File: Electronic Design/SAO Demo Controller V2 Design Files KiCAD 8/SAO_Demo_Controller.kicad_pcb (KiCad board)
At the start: 2 copper layers, 38.1 x 50.8 mm, 10 parts, among them U1 RP2040-Zero, X1 SAO_conn, X2 SAO_conn, X5 QWIIC, X6 QWIIC

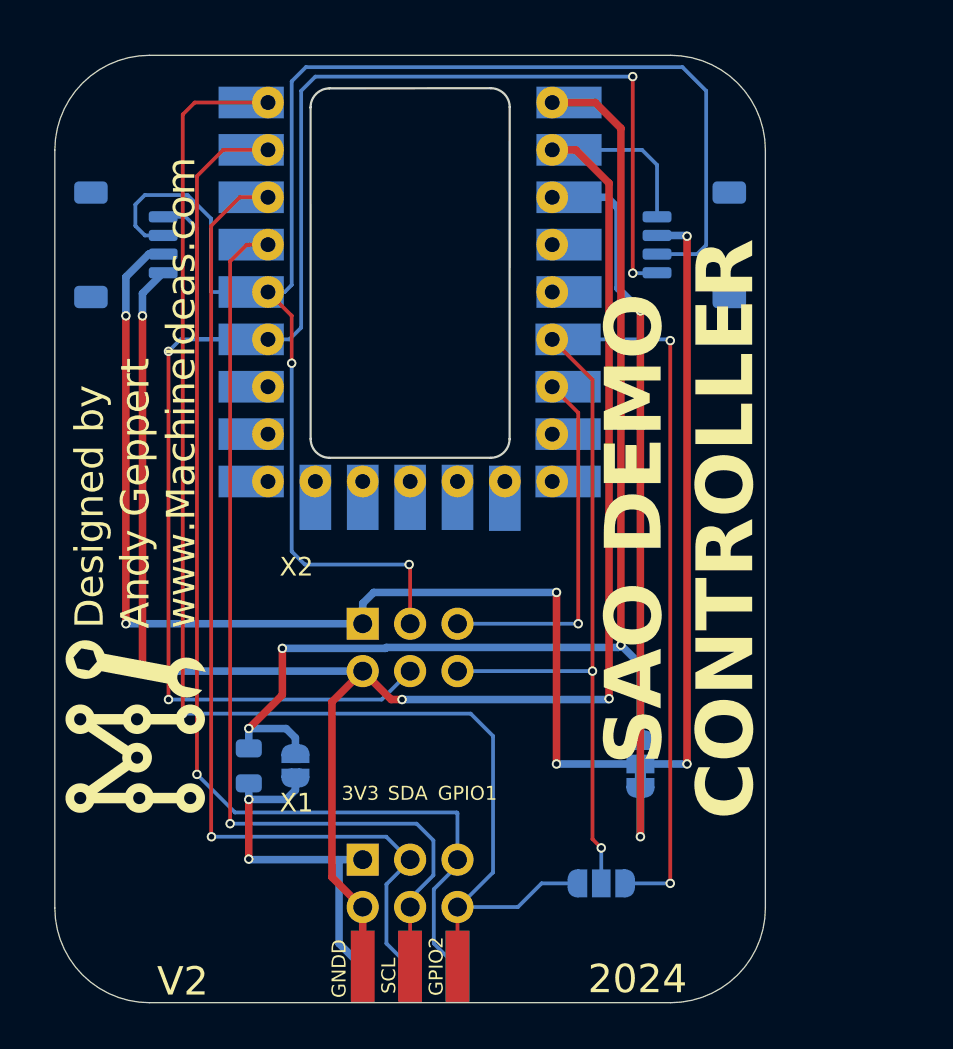
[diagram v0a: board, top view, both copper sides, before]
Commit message: Update V2 schematics, docs, renders
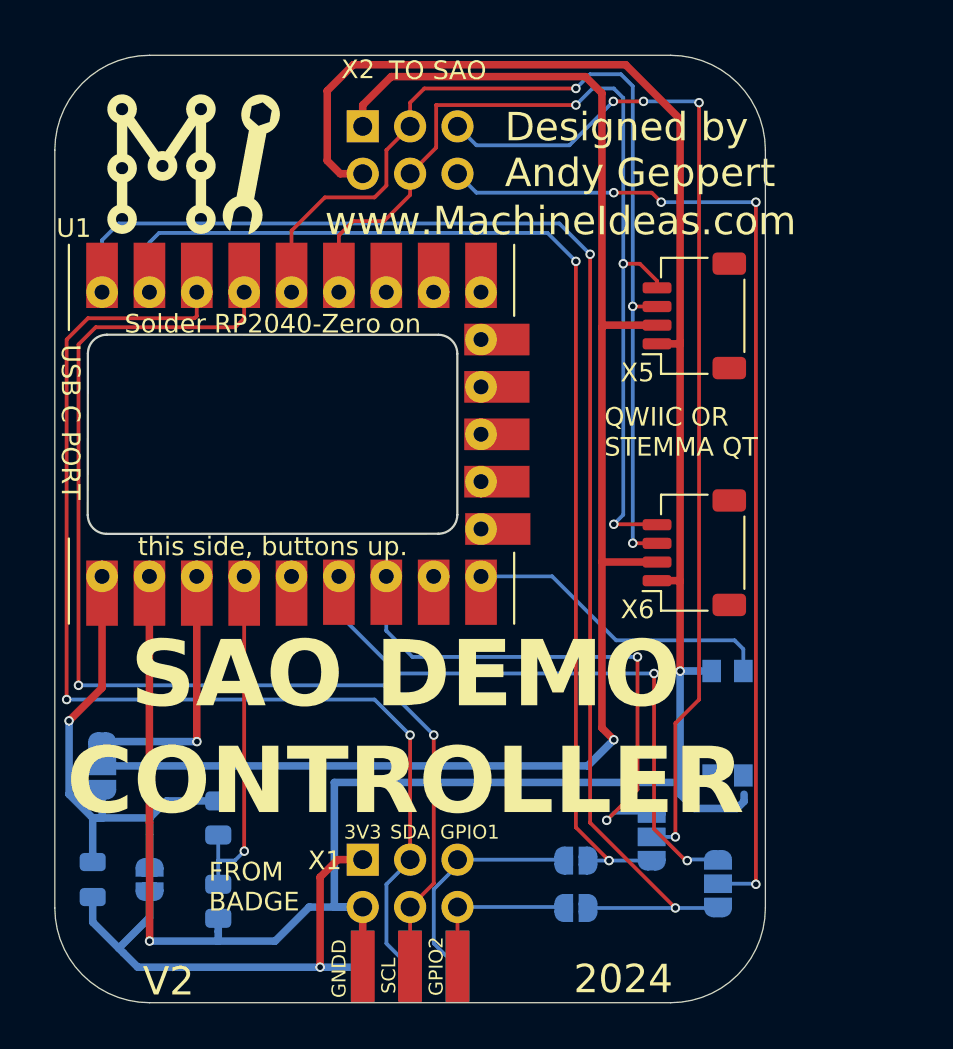
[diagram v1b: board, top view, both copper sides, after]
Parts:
- added JP2: SJ_GPIO1_PASSTHRU, Jumper:SolderJumper-2_P1.3mm_Open_RoundedPad1.0x1.5mm, B.Cu at (116.4, 157.4)
- added JP3: SJ_GPIO2_PASSTHRU, Jumper:SolderJumper-2_P1.3mm_Open_RoundedPad1.0x1.5mm, B.Cu at (116.4, 159.9)
- added JP5: SolderJumper_3_Open, Jumper:SolderJumper-3_P1.3mm_Open_RoundedPad1.0x1.5mm_NumberLabels, B.Cu at (120.5, 156.1)
- added L1: ~, Andy_Footprint_Library:Machine_Ideas_logo, B.Cu at (120.1, 123.5)
- added R1: 4K7, Resistor_SMD:R_0805_2012Metric, B.Cu at (97.2, 155.1)
- added R2: 4K7, Resistor_SMD:R_0805_2012Metric, B.Cu at (97.2, 159.6)
- added S1: 434331045822, Andy_Footprint_Library:Button_Wurth_4343X10458XX, B.Cu at (124.5, 150.0)
- JP1: value SolderJumper_2_Open -> SJ_VIN_VUSB_PASSTHRU
- U1, X5, X6: moved to F.Cu
- moved X5 30.7 mm to (122.8, 128.2)
- moved L1 29.6 mm to (96.3, 120.3), turned to 0 degrees
- moved JP4 28.9 mm to (91.0, 152.3), turned to -90 degrees
- moved X2 26.7 mm to (107.5, 119.3)
- moved X6 16.5 mm to (122.8, 140.9), turned to 90 degrees
- moved D1 10.4 mm to (90.5, 158.4)
- moved U1 9.92 mm to (101.2, 134.5), turned to 90 degrees
- moved JP1 9.92 mm to (93.5, 158.4)
- moved JP6 6.26 mm to (124.0, 158.6), turned to 90 degrees
- renumbered JP2 to JP4, JP3 to JP6
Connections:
- D1 pad 1: /5V -> /5VUSB
- JP1 pad 2: /5V -> /5VUSB
- JP4 pad 3: /5V -> /5VUSB
- JP6 pad 1: /BRX_SAOTX -> /GP0
- U1 pad 1: /5V -> /GP1
- U1 pad 10: /BRX_SAOTX -> unconnected-(U1-GP10-Pad10)_1
- U1 pad 11: /BTX_SAORX -> unconnected-(U1-GP11-Pad11)
- U1 pad 12: /SDA_IN -> unconnected-(U1-GP12-Pad12)
- U1 pad 13: /SCL_IN -> unconnected-(U1-GP13-Pad13)
- U1 pad 14: /SAO_GPIO1 -> Net-(U1-GP14)
- U1 pad 15: /SAO_GPIO1 -> unconnected-(U1-GP15-Pad15)_1
- U1 pad 2: GND -> /SDA_IN
- U1 pad 3: /3V3 -> /SCL_IN
- U1 pad 4: unconnected-(U1-GP29-Pad4) -> /SDA_OUT
- U1 pad 5: unconnected-(U1-GP28-Pad5) -> /SCL_OUT
- U1 pad 6: /SAO_GPIO2_GP27 -> unconnected-(U1-GP6-Pad6)
- U1 pad 7: /SAO_GPIO1 -> unconnected-(U1-GP7-Pad7)_1
- X2 pad 3: /SAO_GPIO1 -> /SDA_OUT
- X2 pad 4: /SAO_GPIO1 -> /SCL_OUT
- X5 pad 3: /SAO_GPIO1 -> /SDA_OUT
- X5 pad 4: /SAO_GPIO1 -> /SCL_OUT
- X6 pad 3: /SAO_GPIO1 -> /SDA_OUT
- X6 pad 4: /SAO_GPIO1 -> /SCL_OUT
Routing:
- net /SAO_GPIO1: track 197.7 -> 55.5 mm, vias 7 -> 4
- net /GP0: track 0.00 -> 73.2 mm, vias 0 -> 2
- net /5V: track 65.4 -> 0.00 mm, vias 3 -> 0
- net /BRX_SAOTX: track 74.2 -> 8.90 mm, vias 1 -> 0
- net /GP1: track 0.00 -> 62.7 mm, vias 0 -> 2
- net /SDA_OUT: track 0.00 -> 54.3 mm, vias 0 -> 3
- net /SCL_OUT: track 0.00 -> 51.7 mm, vias 0 -> 3
- net /BTX_SAORX: track 60.6 -> 12.2 mm, vias 1 -> 0
- net GND: track 104.0 -> 134.2 mm, vias 4 -> 2
- net /SAO_GPIO1_GP26: track 0.00 -> 29.0 mm, vias 0 -> 2
- net /5VUSB: track 0.00 -> 28.3 mm, vias 0 -> 1
- net /3V3: track 40.6 -> 13.9 mm, vias 2 -> 1
- net Net-(U1-GP29/ADC3): track 0.00 -> 19.0 mm, vias 0 -> 1
- net /SAO_GPIO2: track 37.5 -> 55.3 mm, vias 2 -> 4
- net Net-(U1-GP14): track 0.00 -> 16.9 mm
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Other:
- board text added: "3V3"
- board text added: "5V"
- board text added: "Designed by Andy Geppert"
- board text added: "FROM BADGE"
- board text added: "QWIIC OR STEMMA QT"
- board text added: "Solder RP2040-Zero on"
- board text added: "TO SAO"
- board text added: "this side, buttons up."
- board text added: "www.MachineIdeas.com"
- board text removed: "Designed by Andy Geppert www.MachineIdeas.com"
- board text removed: "Solder RP2040-Zero on this side."
